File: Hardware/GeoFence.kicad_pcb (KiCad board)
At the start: 2 copper layers, 78 parts, among them J1 U.FL, J2 microB, J3 AVR_SPI_PROG_3X2PTH, J4 CONN_04, J5 CONN_04, J6 CONN_04X2, Q1 8/16/20MHz, Q2 2.5A/30V, U1 TITAN X1 GPS, U2 74LVC1G08SE, U3 CH340G, U4 AP2112K-3.3V, U5 ATMEGA328, U6 MCP73831, Y1 12MHz

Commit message: Moved Reference labels to drwg layer
The board layout is beginning to take form
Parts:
- removed JP1, JP3, JP4, JP7: STAND-OFF, Hardware:STAND-OFF
- removed LED1: Red, LEDs:LED_0603
- removed R5: 10k, Resistors_SMD:R_0603
- C5, C6: footprint Capacitors_Tantalum_SMD:CP_Tantalum_Case-A_EIA-3216-18_Reflow -> Capacitors_SMD:C_0603
- LOGO1: moved to F.Cu
- U4: footprint DiscreteSemi:SparkFun-DiscreteSemi-SC70-6 -> IC:SOT23-5
- moved U$1 163.6 mm to (154.7, 135.1)
- moved R19 118.6 mm to (150.4, 89.4), turned to 90 degrees
- moved R16 118.2 mm to (159.8, 86.9), turned to 90 degrees
- moved R17 113.9 mm to (151.9, 84.1), turned to 90 degrees
- moved D10 113.9 mm to (160.4, 89.7), turned to 180 degrees
- moved Q2 111.1 mm to (160.0, 82.5), turned to 270 degrees
- moved POWER 104.7 mm to (146.1, 95.2), turned to 90 degrees
- moved CHG 100.0 mm to (150.4, 86.9), turned to 270 degrees
- moved U6 93.7 mm to (154.7, 84.1)
- moved C15 93.6 mm to (157.0, 86.9), turned to 270 degrees
- moved C11 86.5 mm to (152.4, 95.2), turned to 90 degrees
- moved R20 76.9 mm to (149.1, 95.2), turned to 90 degrees
- moved C6 76.4 mm to (161.0, 95.2), turned to 90 degrees
- moved C5 75.5 mm to (153.4, 89.4), turned to 270 degrees
- moved JP8 75.1 mm to (154.4, 79.8)
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- renumbered D11 to CHG, D12 to POWER, D4 to RX, D3 to TX
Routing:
- net /BACKUP: track 13.9 -> 0.00 mm
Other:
- board outline added: 30.5 x 65 mm
- board text added: "A0"
- board text added: "A1"
- board text added: "A2"
- board text added: "A3"
- board text added: "A4"
- board text added: "A5"
- board text added: "A6"
- board text added: "A7"
- board text added: "GND"
- board text added: "ISP"
- board text added: "SIG"
- board text added: "STATUS"
- board text added: "ZONE 1"
- board text added: "ZONE 2"
- board text added: "ZONE 3"
- board text added: "ZONE 4"
- board text removed: "0.8mm PCB for microstrip"
- board text removed: "ANT"

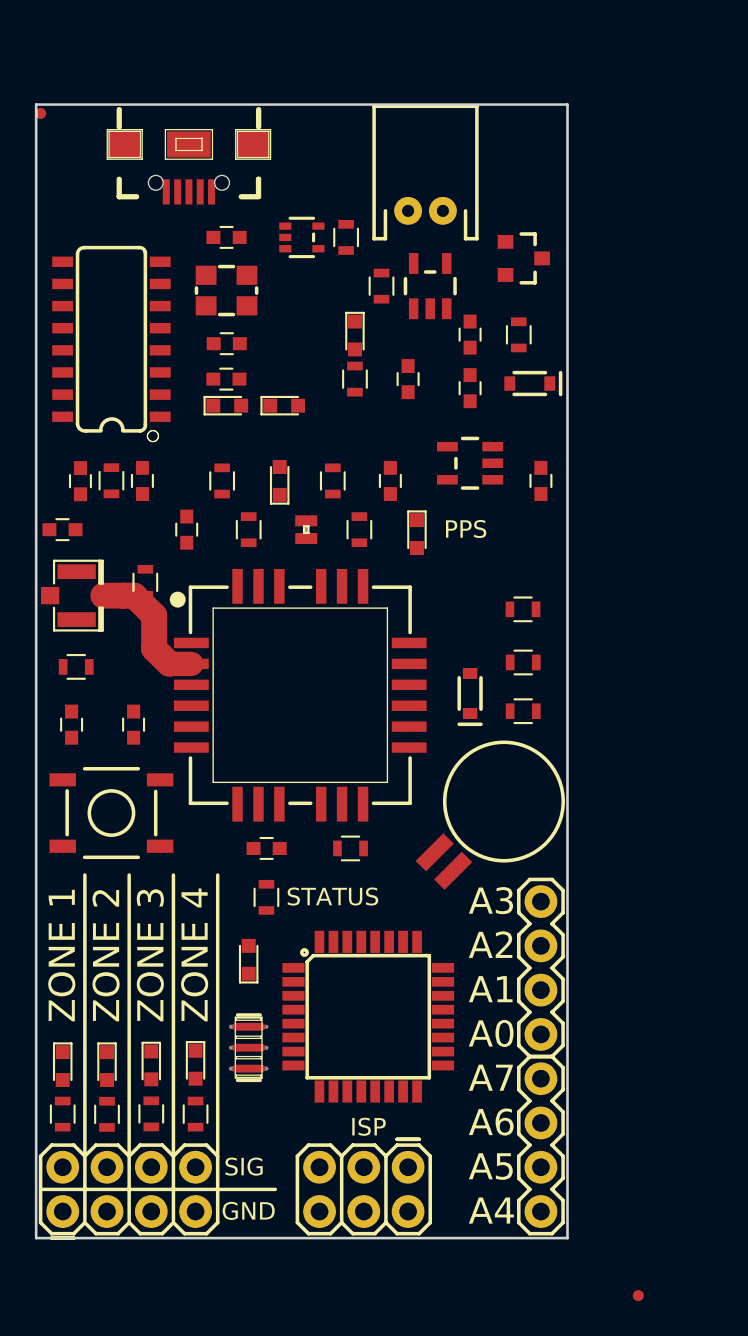
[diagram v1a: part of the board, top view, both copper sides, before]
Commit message: Routing
Started Routing
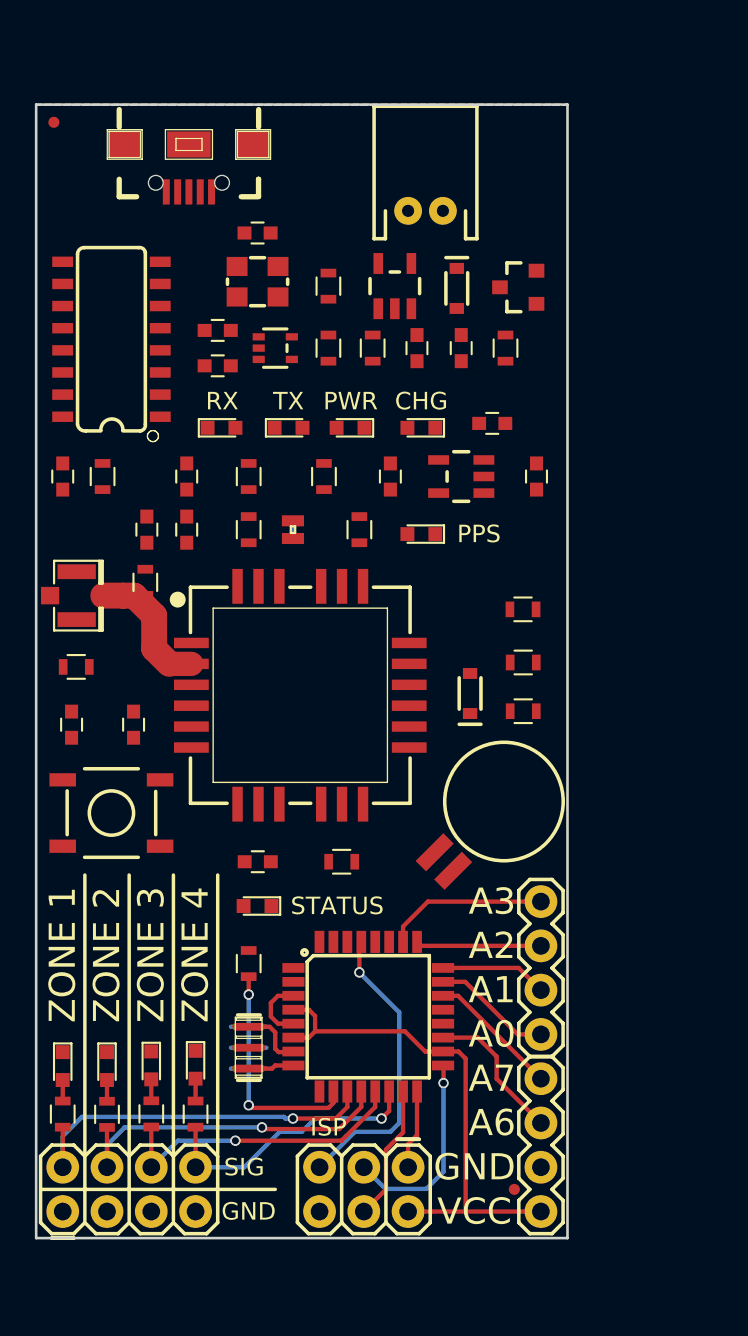
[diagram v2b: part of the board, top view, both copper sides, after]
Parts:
- removed CHG, TX: Yellow, LEDs:LED_0603
- removed POWER: RED, LEDs:LED_0603
- removed RX: GREEN, LEDs:LED_0603
- added D11: Yellow, LEDs:LED_0603, F.Cu at (154.2, 92.2)
- added D12: RED, LEDs:LED_0603, F.Cu at (150.1, 92.2)
- added D3: Yellow, LEDs:LED_0603, F.Cu at (146.6, 92.2)
- added D4: GREEN, LEDs:LED_0603, F.Cu at (142.7, 92.2)
- moved JP2 9.37 mm to (159.5, 135.9)
- moved D10 6.88 mm to (156.2, 84.2), turned to 270 degrees
- moved U2 6.53 mm to (145.8, 87.6)
- moved R1 6.43 mm to (148.8, 87.6)
- moved C12 4.84 mm to (138.4, 98.0), turned to 90 degrees
- moved R15 3.93 mm to (144.3, 122.9), turned to 270 degrees
- moved D9 3.13 mm to (144.8, 119.6), turned to 180 degrees
- moved R17 3.05 mm to (148.8, 84.1)
- moved C9 2.55 mm to (140.7, 95.0)
- moved C7 2.39 mm to (158.2, 91.9), turned to 0 degrees
- moved R19 2.05 mm to (151.4, 87.6), turned to 270 degrees
- moved U6 2.03 mm to (152.7, 84.1)
- moved C5 1.85 mm to (153.9, 87.6), turned to 90 degrees
- moved Y1 1.85 mm to (144.8, 83.8)
- moved C2 1.80 mm to (144.8, 81.0)
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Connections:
- J3 pad 2: VCC -> +3V3
- J4 pad 1: /A4 -> +3V3
- J4 pad 2: /A5 -> GND
- J6 pad 1: Net-(J6-Pad1) -> GND
- J6 pad 3: Net-(J6-Pad3) -> GND
- J6 pad 5: Net-(J6-Pad5) -> GND
- R1 pad 2: VCC -> +3V3
- U2 pad 5: VCC -> +3V3
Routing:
- net +3V3: track 0.00 -> 29.3 mm
- net /D7: track 0.00 -> 22.1 mm, vias 0 -> 1
- net /D8: track 0.00 -> 20.0 mm, vias 0 -> 1
- net /D9: track 0.00 -> 17.5 mm, vias 0 -> 1
- net /ATRESET: track 0.00 -> 17.0 mm, vias 0 -> 1
- net /D10: track 0.00 -> 15.9 mm, vias 0 -> 1
- net /STATUS: track 0.00 -> 13.1 mm, vias 0 -> 2
- net /SCK: track 0.00 -> 11.9 mm, vias 0 -> 1
- net /A3: track 0.00 -> 9.38 mm
- net /A6: track 0.00 -> 8.39 mm
- net /MOSI: track 0.00 -> 7.82 mm
- net /A7: track 0.00 -> 7.58 mm
- net /A2: track 0.00 -> 7.20 mm
- net /A0: track 0.00 -> 6.86 mm
- net /A1: track 0.00 -> 6.14 mm
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- added copper zone on B.Cu, net GND
- added copper zone on F.Cu, net GND
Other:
- board text added: "CHG"
- board text added: "PWR"
- board text added: "RX"
- board text added: "TX"
- board text added: "VCC"
- board text removed: "A4"
- board text removed: "A5"

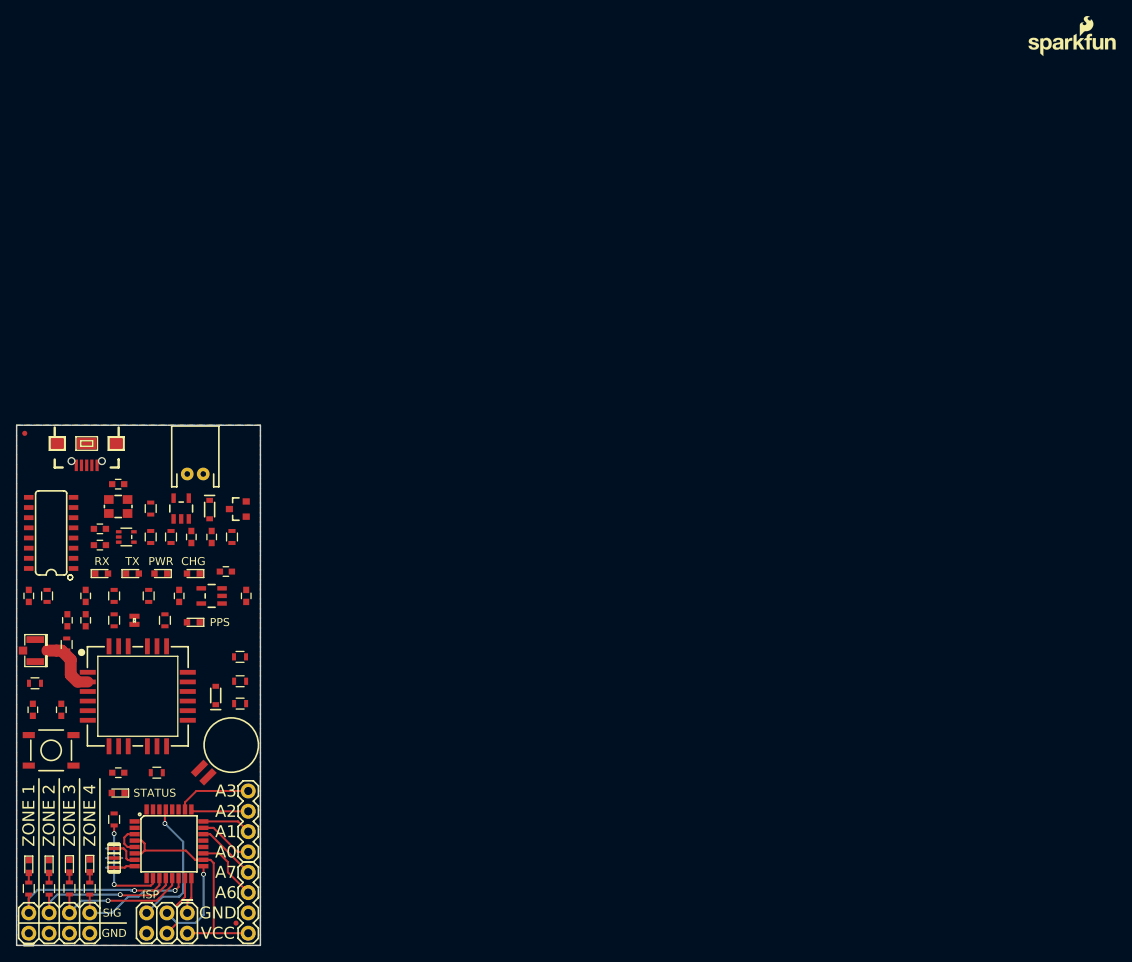
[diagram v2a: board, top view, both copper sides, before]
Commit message: Ready for Review
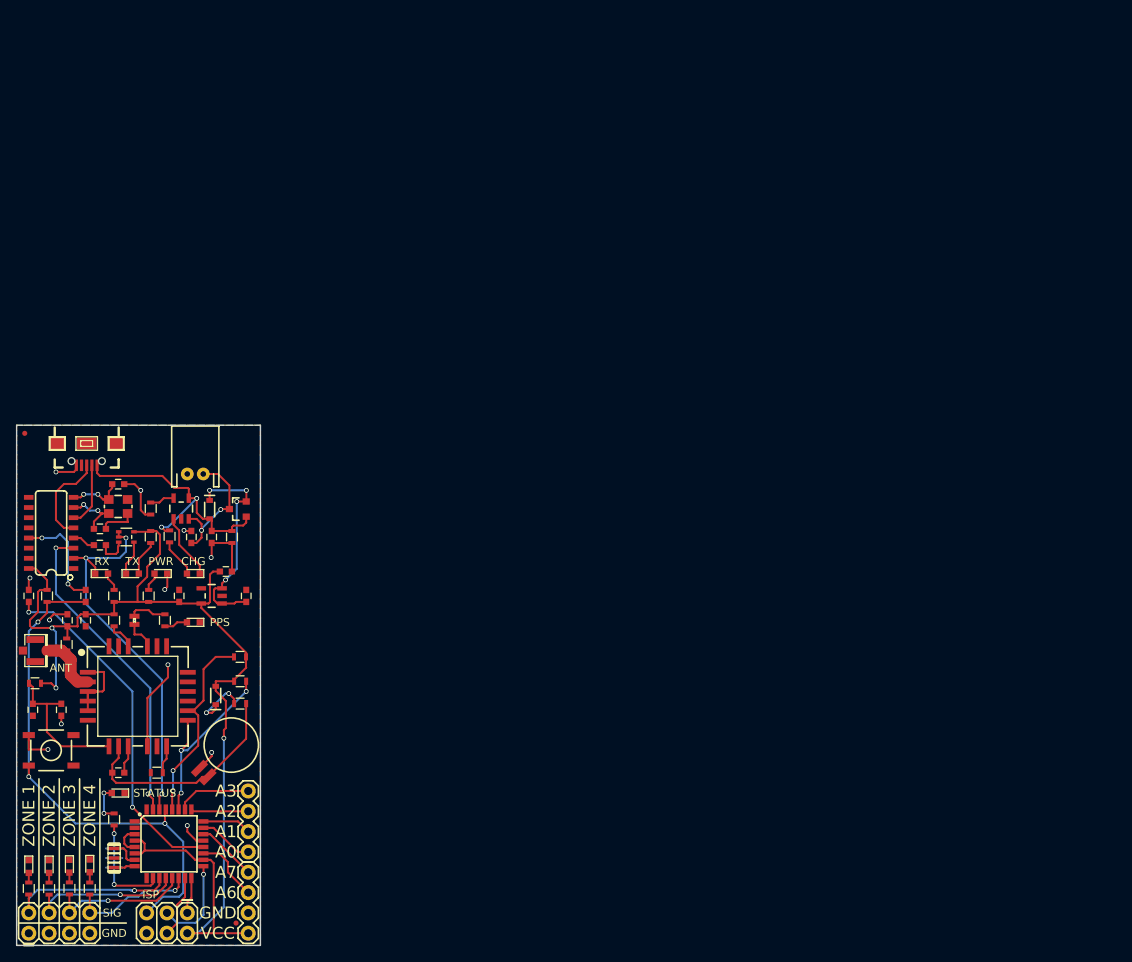
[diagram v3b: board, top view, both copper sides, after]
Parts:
- removed LOGO1: SFE_LOGO_NAME.1_INCH, Aesthetics:SFE_LOGO_NAME_.1
- removed LOGO2: SFE_LOGO_FLAME.1_INCH, Aesthetics:SFE_LOGO_FLAME_.1
- moved U$1 58.3 mm to (134.6, 80.4), turned to 270 degrees
- moved R19 0.20 mm to (151.2, 87.5)
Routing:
- net +3V3: track 29.3 -> 144.3 mm, vias 0 -> 3
- net GND: track 3.71 -> 74.3 mm, vias 0 -> 12
- net /ATRESET: track 17.0 -> 65.5 mm, vias 1 -> 3
- net /RXI: track 0.00 -> 48.1 mm, vias 0 -> 3
- net Net-(C10-Pad1): track 0.00 -> 43.7 mm, vias 0 -> 2
- net /TXO: track 0.00 -> 40.2 mm, vias 0 -> 2
- net +5V: track 0.00 -> 34.4 mm, vias 0 -> 2
- net /BACKUP: track 0.00 -> 28.0 mm
- net Net-(C6-Pad1): track 0.00 -> 26.7 mm, vias 0 -> 4
- net /SCL: track 0.00 -> 24.8 mm, vias 0 -> 2
- net /SDA: track 0.00 -> 24.1 mm, vias 0 -> 3
- net Net-(C13-Pad1): track 0.00 -> 18.3 mm
- net V_BATT: track 0.00 -> 16.7 mm, vias 0 -> 2
- net /DTR: track 0.00 -> 13.3 mm, vias 0 -> 2
- net Net-(J2-PadD+): track 0.00 -> 11.9 mm
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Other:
- rule trace_min: 0.1778 -> 0.2
- board text added: "ANT"
- board text added: "GeoFence"
- board text added: "Reverse Geocache Board"

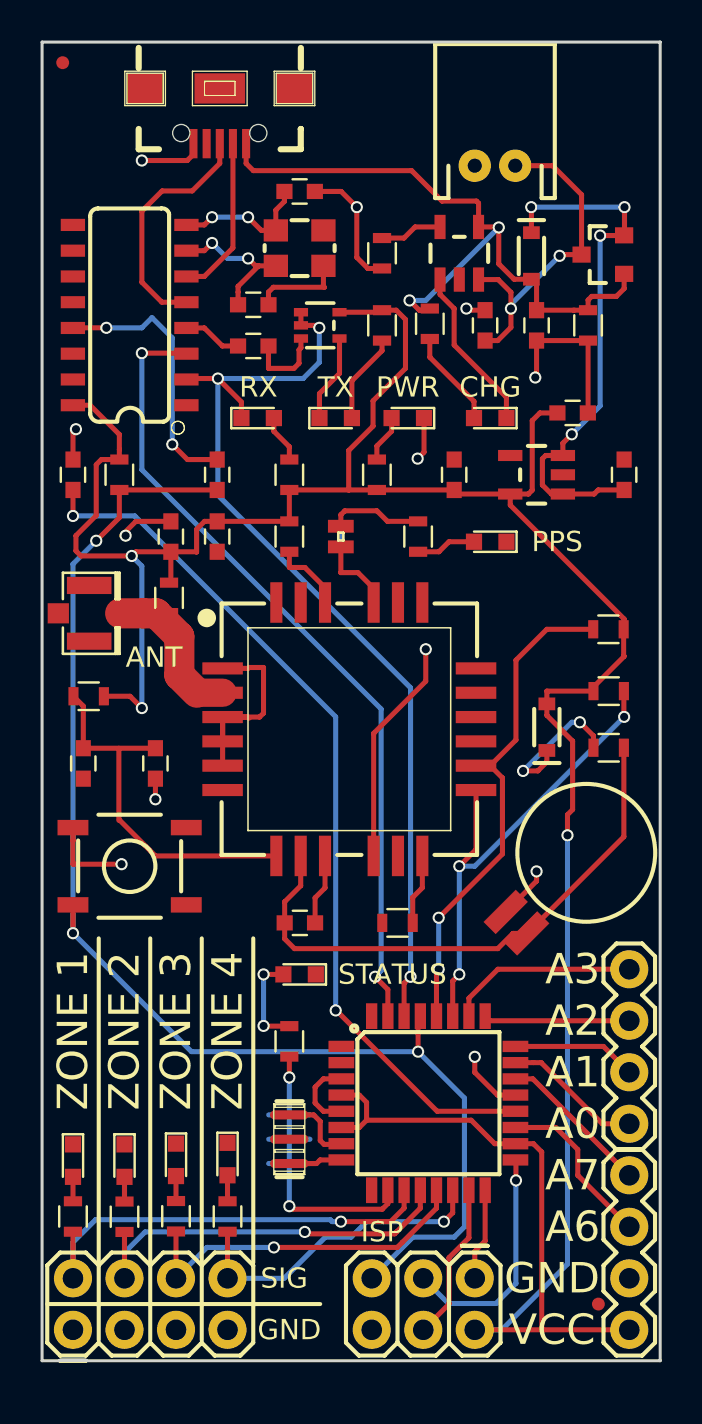
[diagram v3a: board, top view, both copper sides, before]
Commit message: Design Review Changes
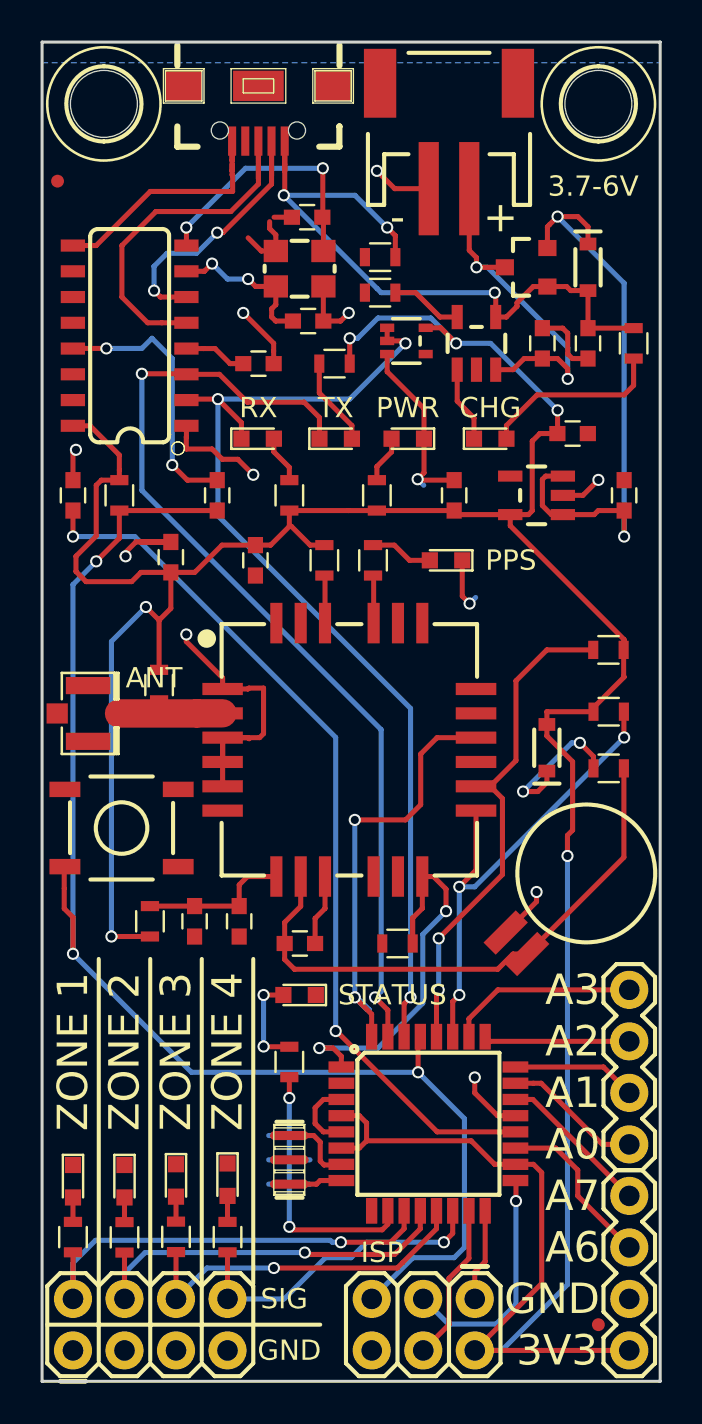
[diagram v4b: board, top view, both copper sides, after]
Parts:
- removed JP5: ~, Jumpers:SMT-JUMPER_2_NC_TRACE_NO-SILK
- removed R19, R20: 1K, Resistors_SMD:R_0603
- added H1: STAND-OFF, STAND-OFF, F.Cu at (159.5, 76.7)
- added H2: STAND-OFF, STAND-OFF, F.Cu at (135.1, 76.7)
- added R18: 1k, Resistors_SMD:R_0603, F.Cu at (148.6, 96.0)
- added R5: 10k, Resistors_SMD:R_0603, F.Cu at (148.8, 84.3)
- D1, D9: value BLUE -> Blue
- D12: value RED -> Red
- D5, D6, D7, D8: value Green -> Blue
- JP8: footprint Connectors:JST-2-PTH -> Connectors:JST-2-SMD
- R1: value 1K -> 1k
- R10, R11, R14, R8: value 330 -> 470
- R16: value 10k -> 2.0k
- R17: value 2.0k -> 1k
- moved R17 13.2 mm to (161.2, 88.5), turned to 270 degrees
- moved FB1 11.5 mm to (137.4, 117.0), turned to 90 degrees
- moved R16 10.4 mm to (148.8, 86.0), turned to 180 degrees
- moved C13 9.52 mm to (139.6, 117.0)
- moved C14 8.81 mm to (141.8, 117.0)
- moved U$1 7.48 mm to (134.6, 87.9)
- moved JP6 5.85 mm to (132.8, 80.5)
- moved J1 4.94 mm to (134.3, 106.8)
- moved U6 4.52 mm to (153.5, 88.5)
- moved L1 4.33 mm to (137.8, 105.4)
- moved U2 4.32 mm to (150.0, 88.4)
- moved Q2 3.84 mm to (156.0, 84.8)
- moved JP8 3.42 mm to (152.1, 77.2)
- moved R1 3.01 mm to (146.5, 89.5), turned to 180 degrees
- moved C5 2.96 mm to (156.8, 88.5)
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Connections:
- D3 pad 1: Net-(D3-Pad1) -> /TXO
- R1 pad 1: Net-(D3-Pad2) -> +3V3
- R1 pad 2: +3V3 -> Net-(D3-Pad2)
- R16 pad 1: GND -> Net-(R16-Pad1)
- R16 pad 2: +5V -> GND
- R17 pad 1: GND -> +5V
- R17 pad 2: Net-(R17-Pad2) -> Net-(D11-Pad2)
- R3 pad 2: Net-(JP5-Pad1) -> /PPS
- U5 pad 1: /D3 -> /WAKE
- U5 pad 32: /D2 -> /INT
- U6 pad 5: Net-(R17-Pad2) -> Net-(R16-Pad1)
- Y1 pad 1: (no net) -> Net-(C2-Pad1)
- Y1 pad 2: Net-(C2-Pad1) -> GND
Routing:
- net /INT: track 0.00 -> 21.8 mm, vias 0 -> 2
- net +3V3: track 144.3 -> 164.1 mm, vias 3 -> 6
- net /WAKE: track 3.50 -> 18.8 mm, vias 0 -> 2
- net Net-(C13-Pad1): track 18.3 -> 7.45 mm
- net /TXO: track 40.2 -> 49.0 mm
- net GND: track 74.3 -> 81.8 mm
- net Net-(C2-Pad1): track 6.93 -> 12.9 mm
- net Net-(J2-PadD+): track 11.9 -> 17.8 mm
- net Net-(J2-PadD-): track 8.02 -> 13.9 mm, vias 0 -> 2
- net Net-(JP5-Pad1): track 4.67 -> 0.00 mm
- net Net-(D11-Pad1): track 8.22 -> 3.75 mm
- net Net-(D3-Pad1): track 4.33 -> 0.00 mm
- net Net-(D11-Pad2): track 4.80 -> 9.07 mm
- net Net-(R16-Pad1): track 0.00 -> 3.55 mm
- net /RXI: track 48.1 -> 51.5 mm
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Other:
- board size 30.5 x 65 mm -> 30.5 x 66 mm
- rule pad_to_mask_clearance: 0.2 -> 0.1
- board text added: "+"
- board text added: "-"
- board text added: "3.7-6V"
- board text added: "3V3"
- board text removed: "VCC"
